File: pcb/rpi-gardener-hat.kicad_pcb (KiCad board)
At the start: 2 copper layers, 65 x 56 mm, 13 parts, among them J1 RPi_GPIO, J2 OLED_RPi, J3 LCD_I2C, J4 DHT22, J5 OLED_Pico, J6 MOISTURE_1, J7 MOISTURE_2, J8 MOISTURE_3, U1 Pico

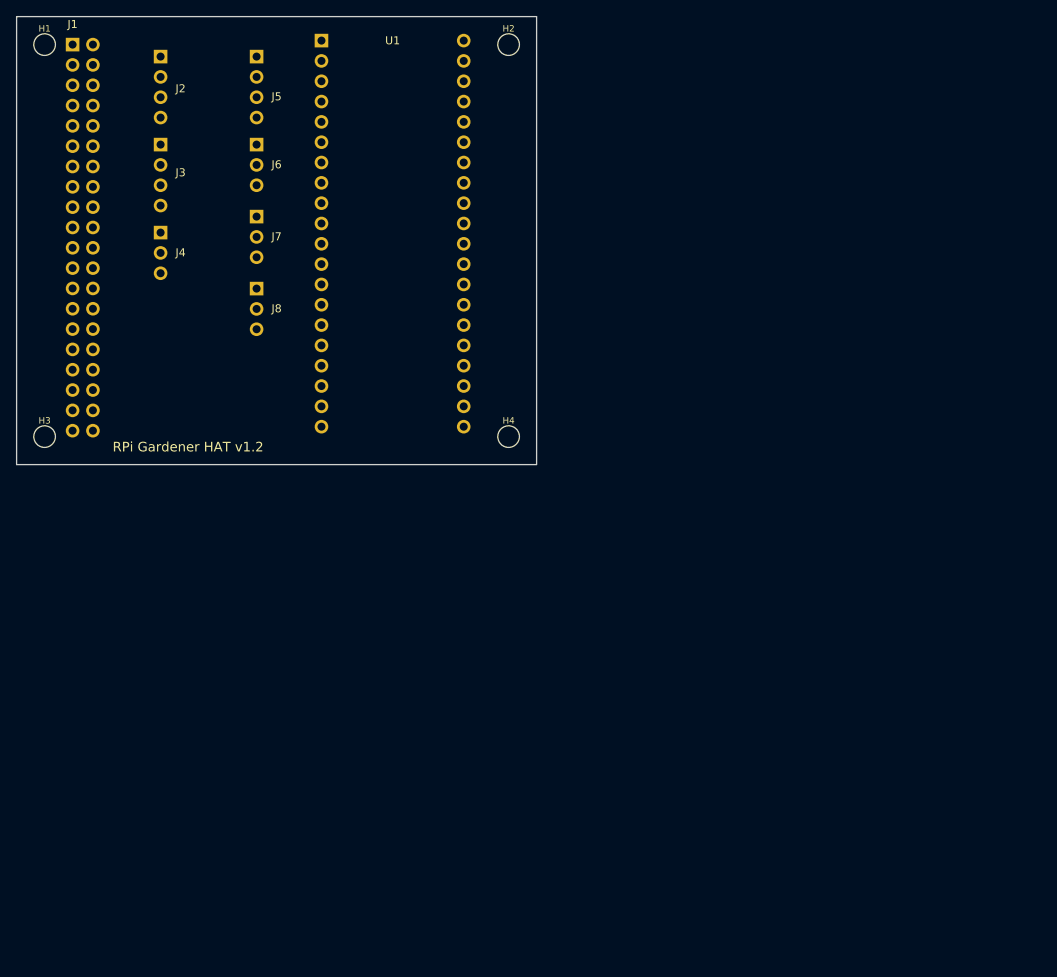
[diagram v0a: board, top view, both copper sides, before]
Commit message: WIP
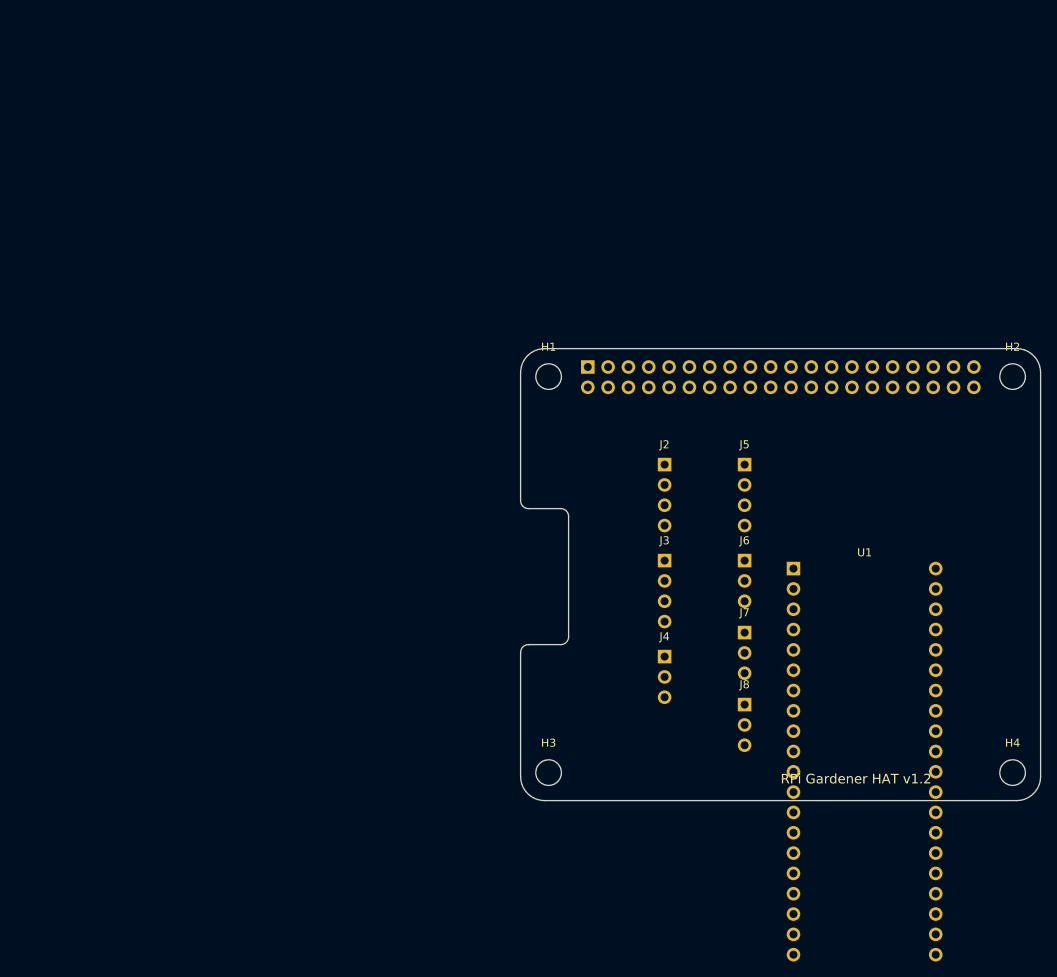
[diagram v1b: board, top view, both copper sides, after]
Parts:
- H1, H2, H3, H4: footprint MountingHole:MountingHole_2.7mm_M2.5 -> MountingHole:MountingHole_3.2mm_M3
- J1: moved to B.Cu
- moved U1 88.5 mm to (120.0, 83.0)
- moved J4 82.3 mm to (95.0, 94.0)
- moved J3 81.7 mm to (95.0, 82.0)
- moved J2 81.1 mm to (95.0, 70.0)
- moved J6 80.2 mm to (105.0, 82.0)
- moved J7 80.2 mm to (105.0, 91.0)
- moved J8 80.2 mm to (105.0, 100.0)
- moved J5 79.5 mm to (105.0, 70.0)
- moved J1 76.0 mm to (85.4, 57.8), turned to 270 degrees
- moved H3 75.7 mm to (80.5, 108.5)
- moved H4 75.7 mm to (138.5, 108.5)
- moved H1 75.4 mm to (80.5, 59.0)
- moved H2 75.4 mm to (138.5, 59.0)
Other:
- board size 65 x 56 mm -> 65 x 56.5 mm
- rule pad_to_mask_clearance: 0 -> 0.051
